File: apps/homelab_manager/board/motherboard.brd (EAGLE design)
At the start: 100 x 80 mm, 50 parts, among them X1 22-23-2021

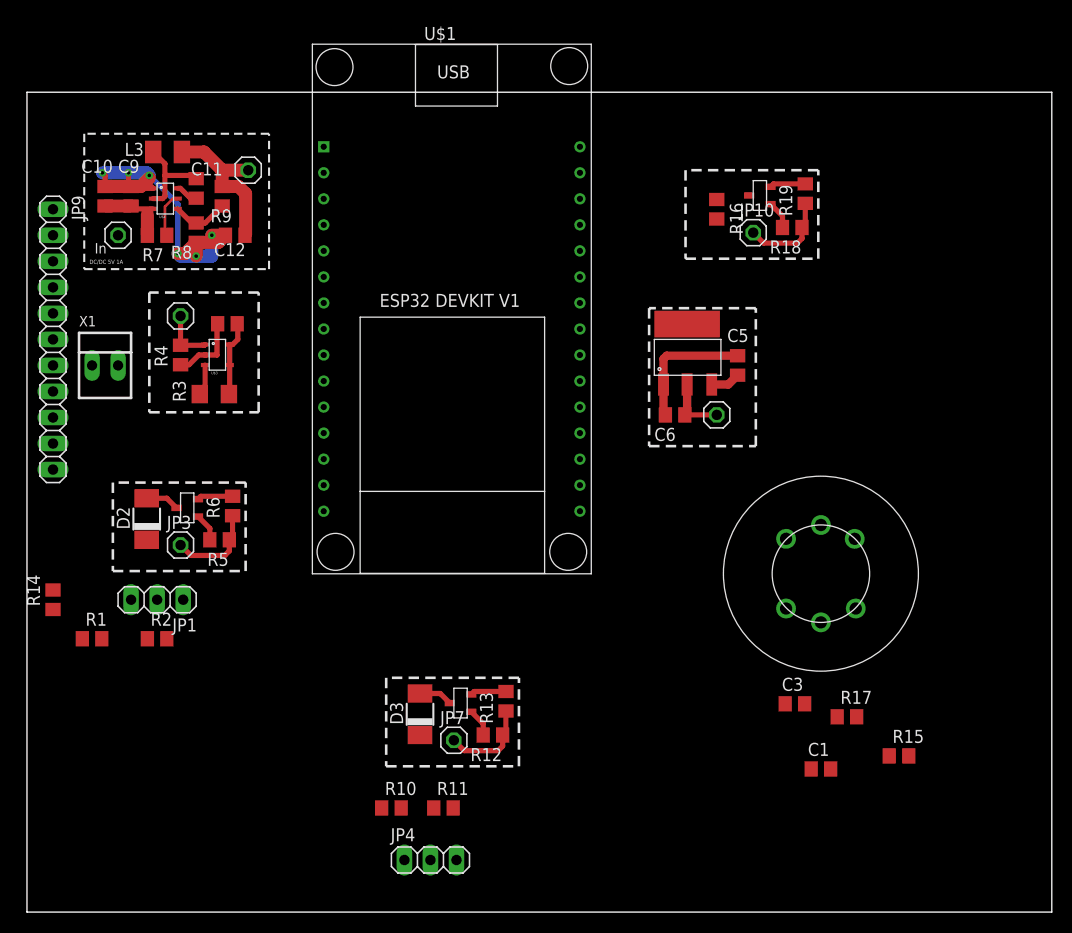
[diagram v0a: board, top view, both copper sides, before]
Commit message: Started main layout
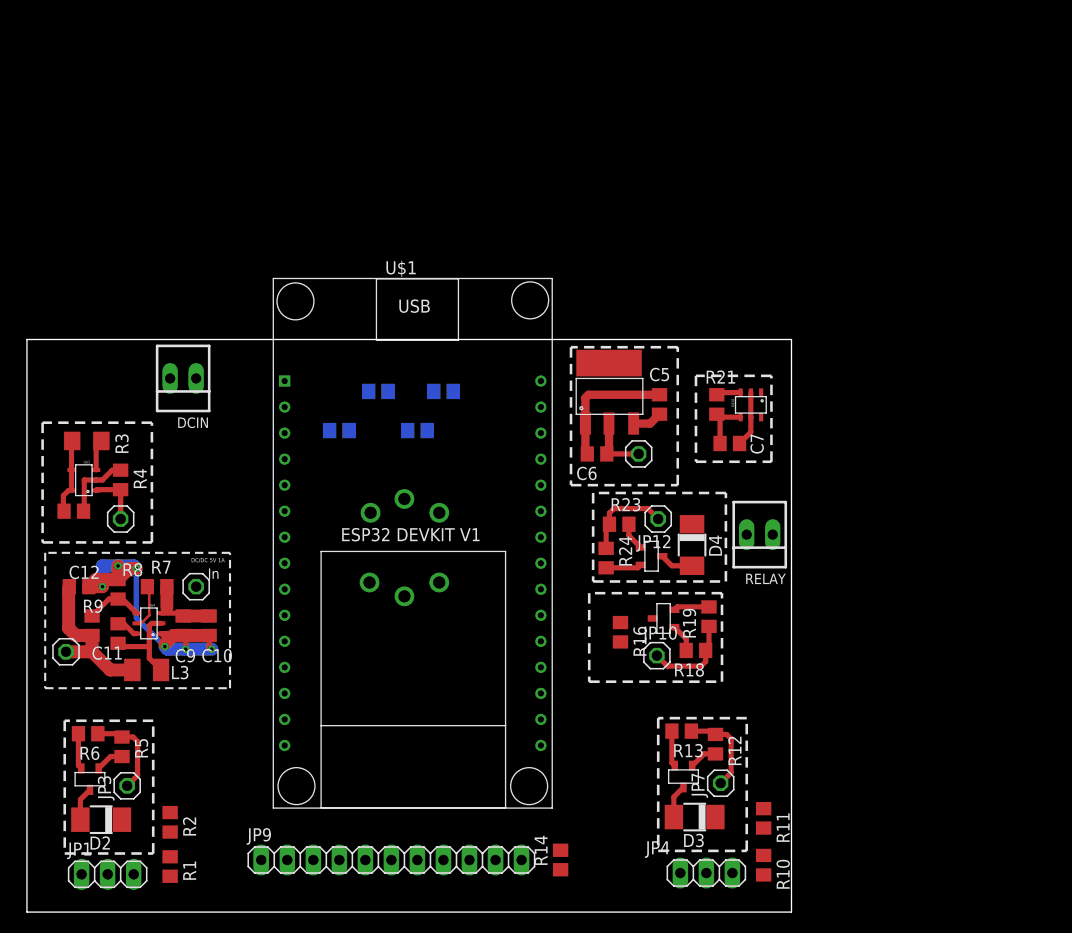
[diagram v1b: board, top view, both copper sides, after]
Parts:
- removed X1: 22-23-2021, con-molex:22-23-2021
- added C7: 100n, rcl:C0805
- added D4: 1N4148, diode:DO-214AC
- added DCIN, RELAY: 22-23-2021, con-molex:22-23-2021
- added JP12: HOMELAB, pinhead:1X01
- added R21, R24: 100k, rcl:R0805
- added R23: 1k, rcl:R0805
- added U$10: TMP101, bzd:SOT23_6_PIN
- added U$11: MGSF1N03L, bzd:SOT23_3_PIN
- moved R15 62.0 mm to (34.3, 50.8), flipped to the bottom
- moved JP9 60.6 mm to (35.6, 5.08), turned to 0 degrees
- moved C1 57.4 mm to (30.5, 47.0), flipped to the bottom
- moved R14 55.7 mm to (52.1, 5.08)
- moved L3 50.6 mm to (11.7, 23.6), turned to 180 degrees
- moved R17 50.4 mm to (38.1, 47.0), flipped to the bottom
- moved JP6 50.2 mm to (3.81, 25.4), turned to 180 degrees
- moved C3 45.9 mm to (40.6, 50.8), flipped to the bottom
- moved U$4 44.5 mm to (12.7, 26.7), turned to 180 degrees
- moved C11 44.1 mm to (8.89, 27.2), turned to 90 degrees
- moved R9 43.8 mm to (6.35, 27.9), turned to 90 degrees
- moved C10 43.1 mm to (17.8, 27.9), turned to 270 degrees
- moved R18 42.3 mm to (65.3, 25.5)
- moved JP10 42.3 mm to (61.5, 25.0)
- moved R16 42.3 mm to (57.9, 27.3)
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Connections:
- new net GND_RELAY: D4.A, RELAY.1, U$11.P$3
- new net HOMELAB_POWER: JP12.1, R23.1, R24.2, U$1.PIN_21
- new net N$13: R23.2, U$11.P$1
- new net TEMPERATURE_ALERT: R21.1, U$1.PIN_25, U$10.3
- net 12V: now also DCIN.2; no longer X1.2
- net 3.3V: now also C7.1, R21.2, U$10.4
- net GND: now also C7.2, DCIN.1, R24.1, U$10.2, U$10.5, U$11.P$2; no longer X1.1
- net I2C_SCL: now also U$10.1
- net I2C_SDA: now also U$10.6
- net LED: now also U$1.PIN_26
- net VIN_REG: now also D4.C, RELAY.2
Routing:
- net HOMELAB_POWER: track 0.00 -> 8.93 mm
- net GND: track 68.5 -> 77.5 mm
- net 3.3V: track 0.00 -> 4.58 mm
- net GND_RELAY: track 0.00 -> 3.29 mm
- net N$13: track 0.00 -> 2.75 mm
- net TEMPERATURE_ALERT: track 0.00 -> 2.41 mm
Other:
- board size 100 x 80 mm -> 74.6 x 55.9 mm
